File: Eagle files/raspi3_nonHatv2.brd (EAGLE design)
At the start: 69.8 x 63.2 mm, 37 parts, among them IC5 PAM8403, K1 PIN20X2

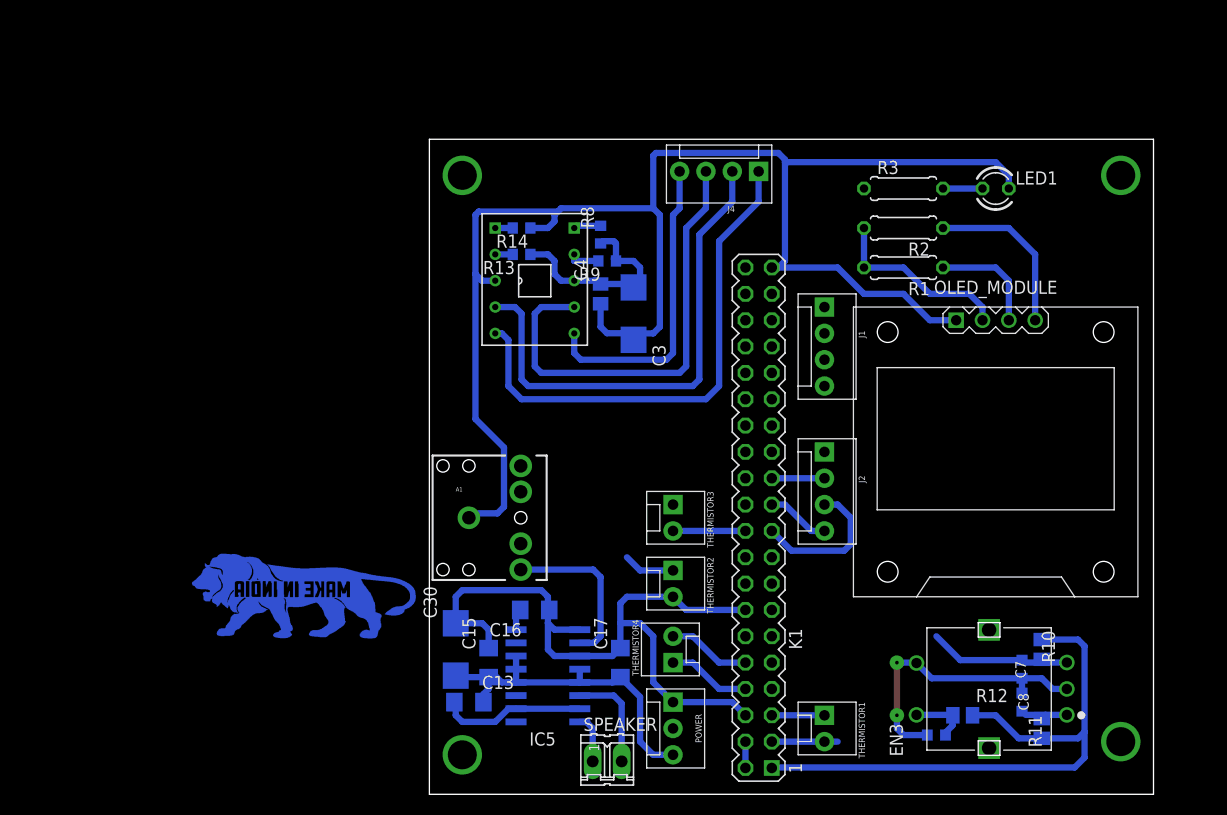
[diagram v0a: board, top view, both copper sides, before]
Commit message: 3-Eagle_final
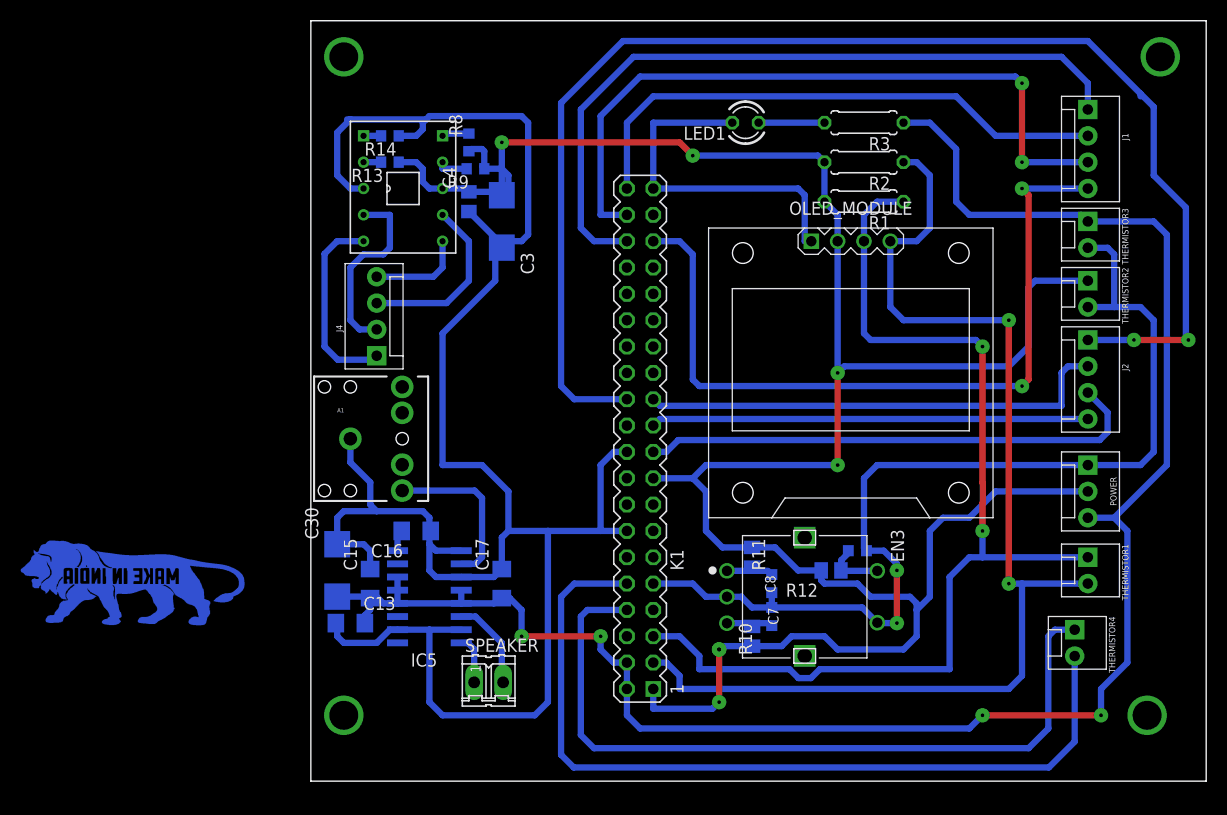
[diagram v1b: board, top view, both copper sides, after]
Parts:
- moved THERMISTOR2 48.8 mm to (74.9, 48.3)
- moved THERMISTOR3 48.4 mm to (74.9, 54.0)
- moved POWER 46.1 mm to (74.9, 30.5)
- moved J4 40.9 mm to (6.35, 41.0), turned to 90 degrees
- moved THERMISTOR4 38.9 mm to (73.7, 14.6), turned to 270 degrees
- moved R11 32.5 mm to (42.5, 21.6), turned to 90 degrees
- moved J1 31.8 mm to (74.9, 64.8)
- moved THERMISTOR1 29.6 mm to (74.9, 21.6)
- moved R10 28.0 mm to (42.5, 14.0), turned to 270 degrees
- moved J2 27.6 mm to (74.9, 42.5)
- moved C8 26.7 mm to (44.5, 19.1), turned to 270 degrees
- moved LED1 25.0 mm to (41.9, 63.5), turned to 180 degrees
- moved C7 24.7 mm to (44.5, 15.9), turned to 90 degrees
- moved EN3 19.9 mm to (47.6, 17.8), turned to 270 degrees
- moved C9 19.3 mm to (52.7, 22.2), turned to 180 degrees
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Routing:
- net +5V: track 36.1 -> 177.0 mm, vias 0 -> 4
- net 0CS0: track 0.00 -> 130.2 mm, vias 0 -> 2
- net +3V3: track 101.2 -> 228.5 mm, vias 0 -> 7
- net SDA: track 22.6 -> 110.6 mm, vias 0 -> 2
- net SCL: track 15.8 -> 102.4 mm, vias 0 -> 2
- net 1MISO: track 0.00 -> 74.3 mm, vias 0 -> 2
- net RX: track 8.04 -> 81.4 mm
- net 1CS0: track 0.00 -> 71.0 mm
- net 1MOSI: track 0.00 -> 68.5 mm, vias 0 -> 2
- net GND: track 268.4 -> 334.3 mm
- net TX: track 8.67 -> 74.2 mm
- net 1SCLK: track 0.00 -> 53.4 mm
- net 0SCLK: track 5.08 -> 45.6 mm
- net 0MISO: track 6.13 -> 42.2 mm
- net 0MOSI: track 14.3 -> 49.2 mm
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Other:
- board size 69.8 x 63.2 mm -> 86.3 x 73.3 mm
